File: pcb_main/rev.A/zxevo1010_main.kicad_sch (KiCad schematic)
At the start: 243 parts, among them J1 Mini-DIN-6, J10 TE 041021-4, J13 Conn_02x05_Odd_Even, J16 MEM2055-00-190-01-A, J17 B2B-XH-A, J18 XHP-2, SXH-002T-P0.6, J2 USB_B_Micro, J22 Conn_02x05_Odd_Even, J3 Mini-DIN-6, J4 PJ-320, J5 Conn_02x05_Odd_Even, J6 Conn_02x30_Row_Letter_First, J8 Conn_02x05_Odd_Even, J9 DB15_Female_HighDensity_Mount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, Q1 BC856, Q2 BC856, Q3 BC856, Q6 BC847, SW1 PB05A, SW3 SW_Push, SW5 SW_Push, SW6 SW_Push, U1 29F040-K, U10 HY5118160, U11 CH340X, U12 LMV358IDR, U13 PCF8583T, U14 LP2985-3.3, U15 74LVC1G04DB, U16 74LVC1G04DB, U17 74LVC1G04DB, U18 74LVC1G04DB, U19 CD4069UBM, U2 EP1K50QC208, U20 74LVC1G04DB, U21 EPM3128ATC100, U22 LP2985-3.3, U23 ADV7125-lqfp48, U24 FT812, U3 Z84C0020FEC, U5 ICS501, U6 ATmega128, U7 HY5118160, U8 1117-3.3, U9 1117-2.5, Y1 14 MHz, Y2 11.059 Mhz, Y3 32768 Hz, Y4 8 MHz

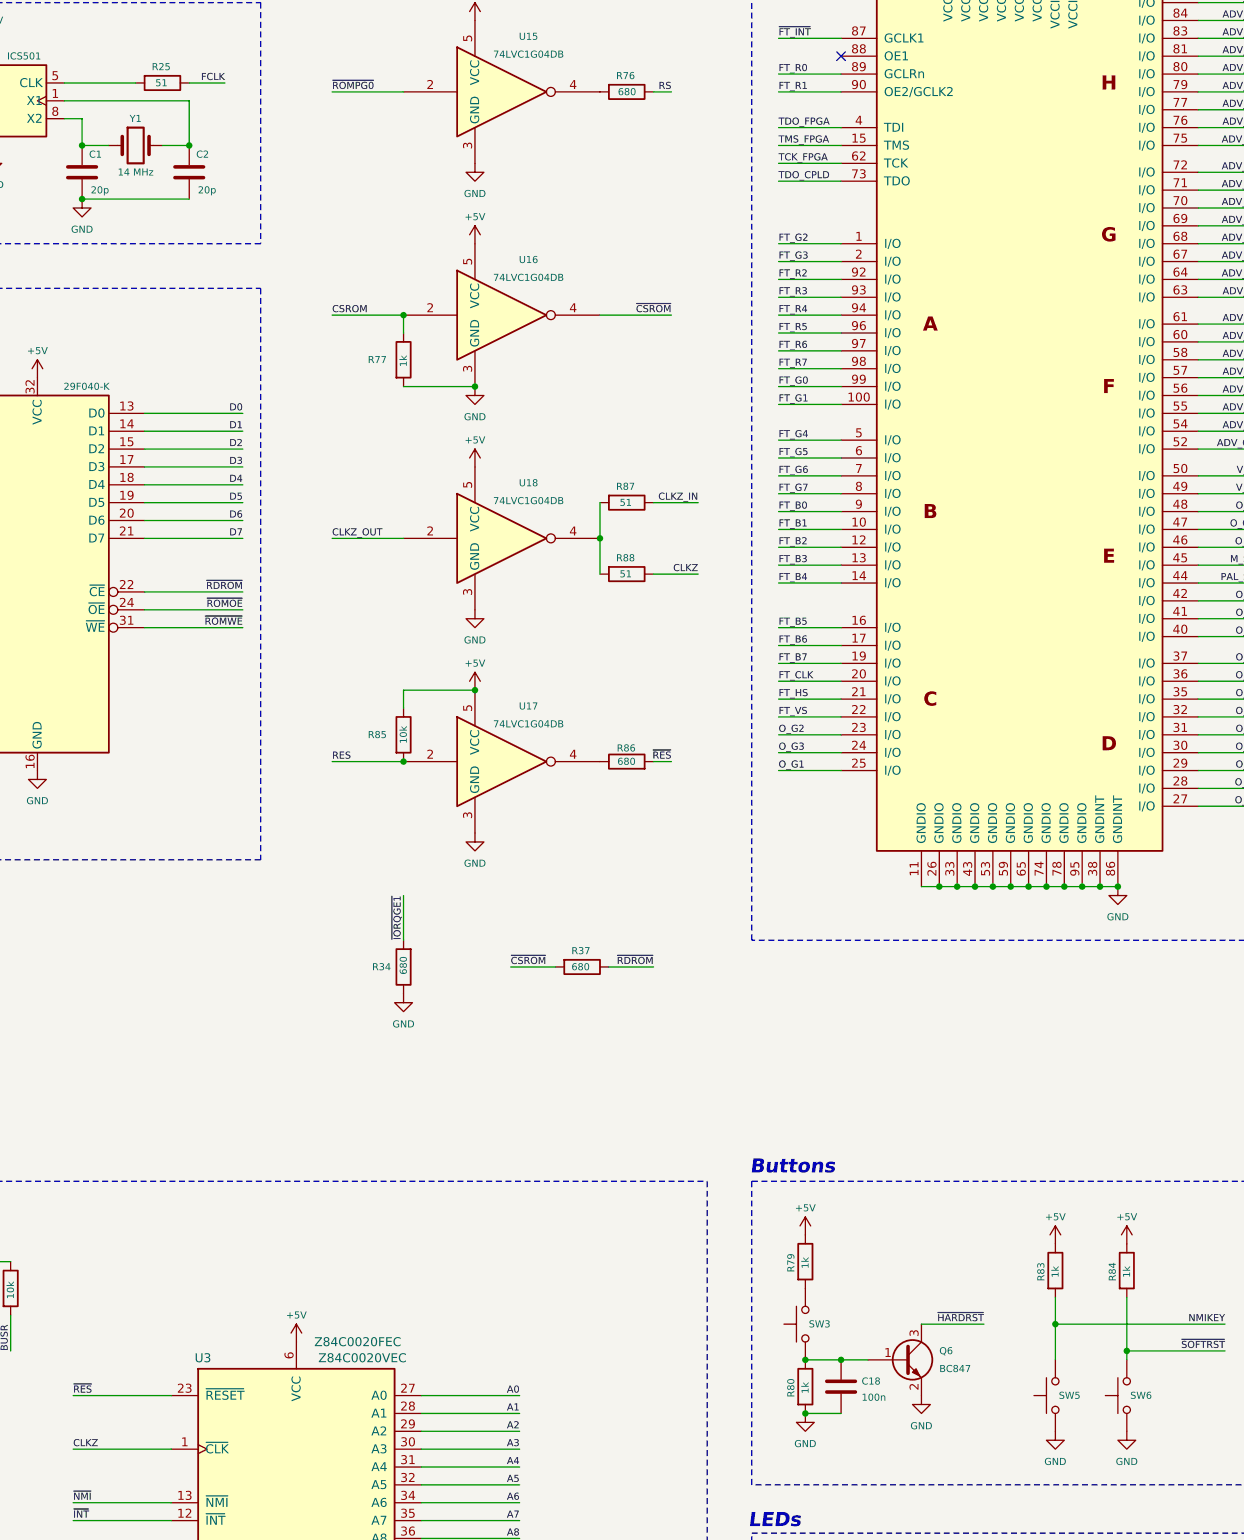
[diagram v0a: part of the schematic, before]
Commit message: wip pcb rev.A
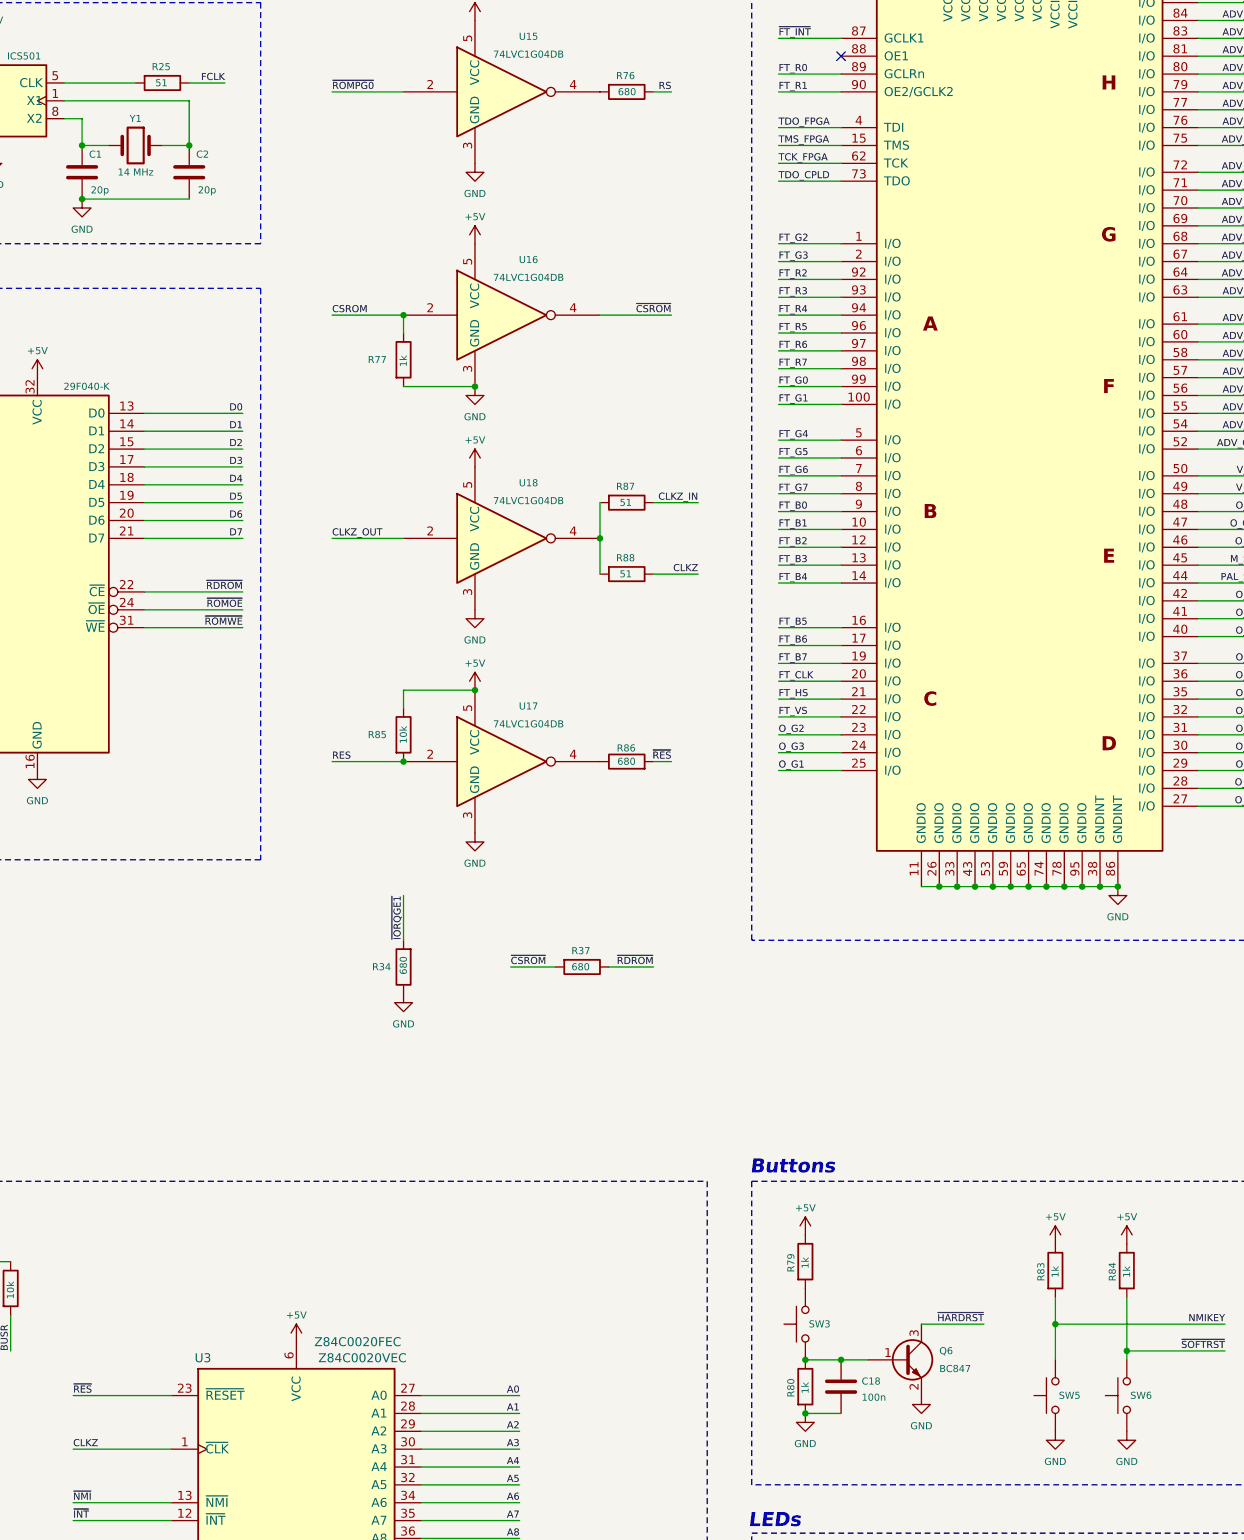
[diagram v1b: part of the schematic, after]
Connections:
- net GND: now also SW5.1, SW6.1; no longer SW5.2, SW6.2
- net NMIKEY: now also SW5.2; no longer SW5.1
- net ~{SOFTRST}: now also SW6.2; no longer SW6.1
- net at C2.2, U5.1 (X1): now also Y1.1; no longer Y1.2
- net at C1.2, U5.8 (X2): now also Y1.2; no longer Y1.1
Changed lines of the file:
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@@
 		(lib_id "Device:Crystal")
 		(at 204.47 129.54 0)
+		(mirror y)
 		(unit 1)
 		(exclude_from_sim no)
@@
 		(lib_id "Switch:SW_Push")
 		(at 345.44 307.34 90)
-		(mirror x)
 		(unit 1)
 		(exclude_from_sim no)
@@
 		)
 		(property "Value" "SW_Push"
-			(at 341.63 309.2449 90)
+			(at 341.63 305.4351 90)
 			(effects
 				(font
@@
 		(lib_id "Switch:SW_Push")
 		(at 335.28 307.34 90)
-		(mirror x)
 		(unit 1)
 		(exclude_from_sim no)
@@
 		)
 		(property "Value" "SW_Push"
-			(at 331.47 309.2449 90)
+			(at 331.47 305.4351 90)
 			(effects
 				(font
